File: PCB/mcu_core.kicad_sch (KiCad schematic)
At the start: 10 parts

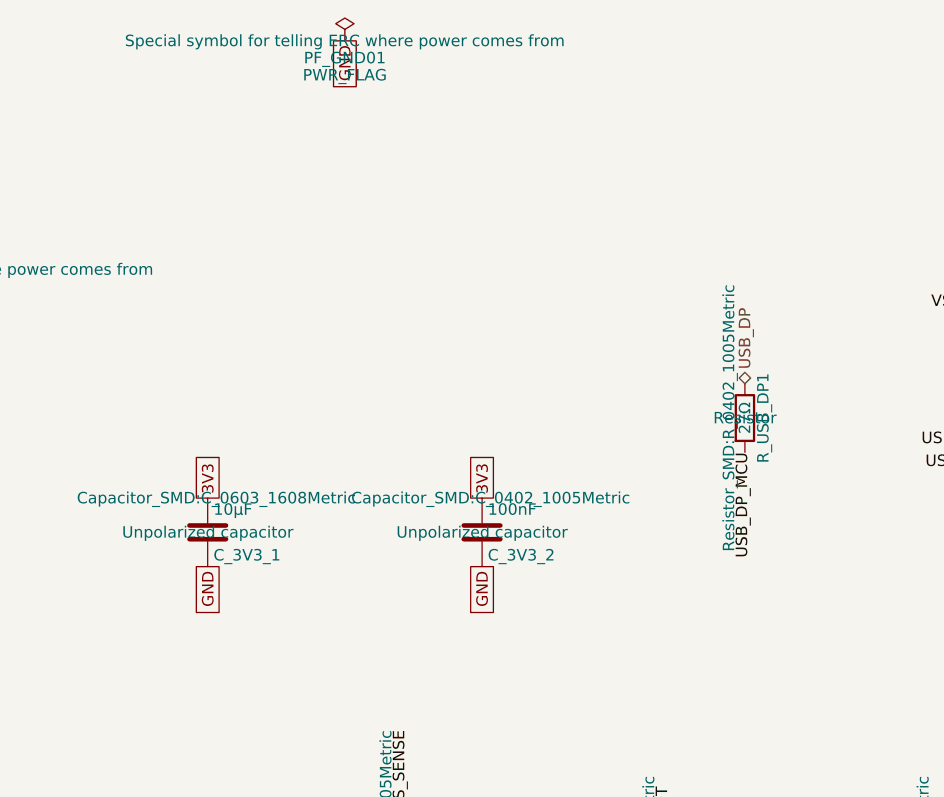
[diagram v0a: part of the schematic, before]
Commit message: task: first validation pass
This is the results post first kicad-happy run.
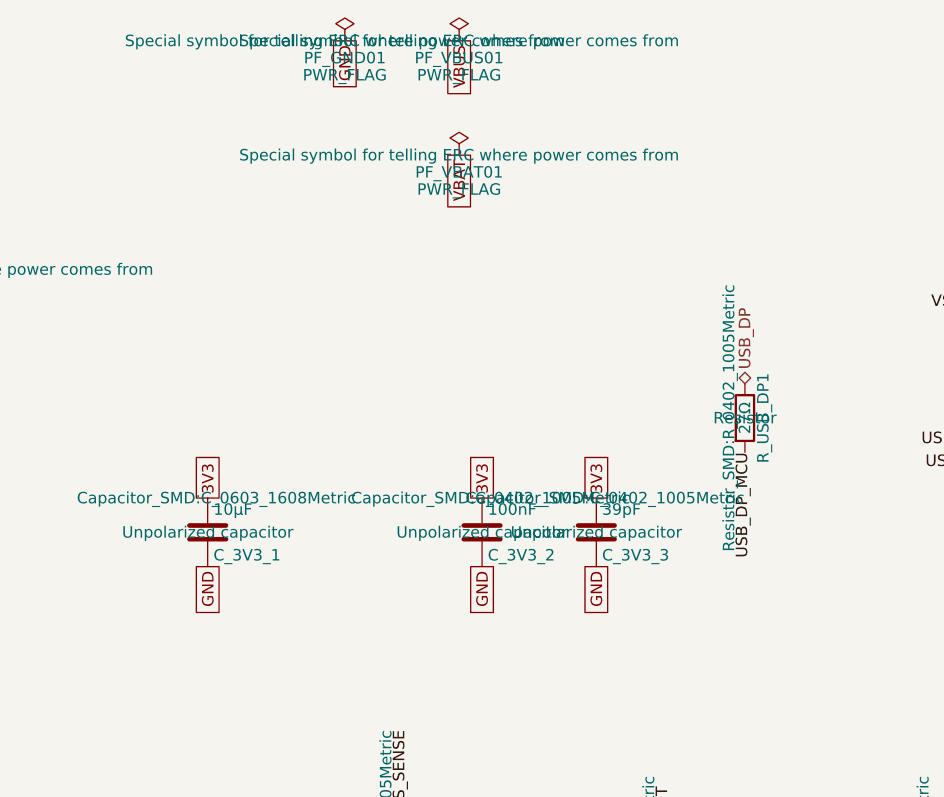
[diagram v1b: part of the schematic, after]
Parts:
- added C_3V3_3: 39pF, Capacitor_SMD:C_0402_1005Metric, symbol Device:C
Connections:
- net 3V3: now also C_3V3_3.1
- net GND: now also C_3V3_3.2
